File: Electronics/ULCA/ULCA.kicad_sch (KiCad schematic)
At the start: 0 parts

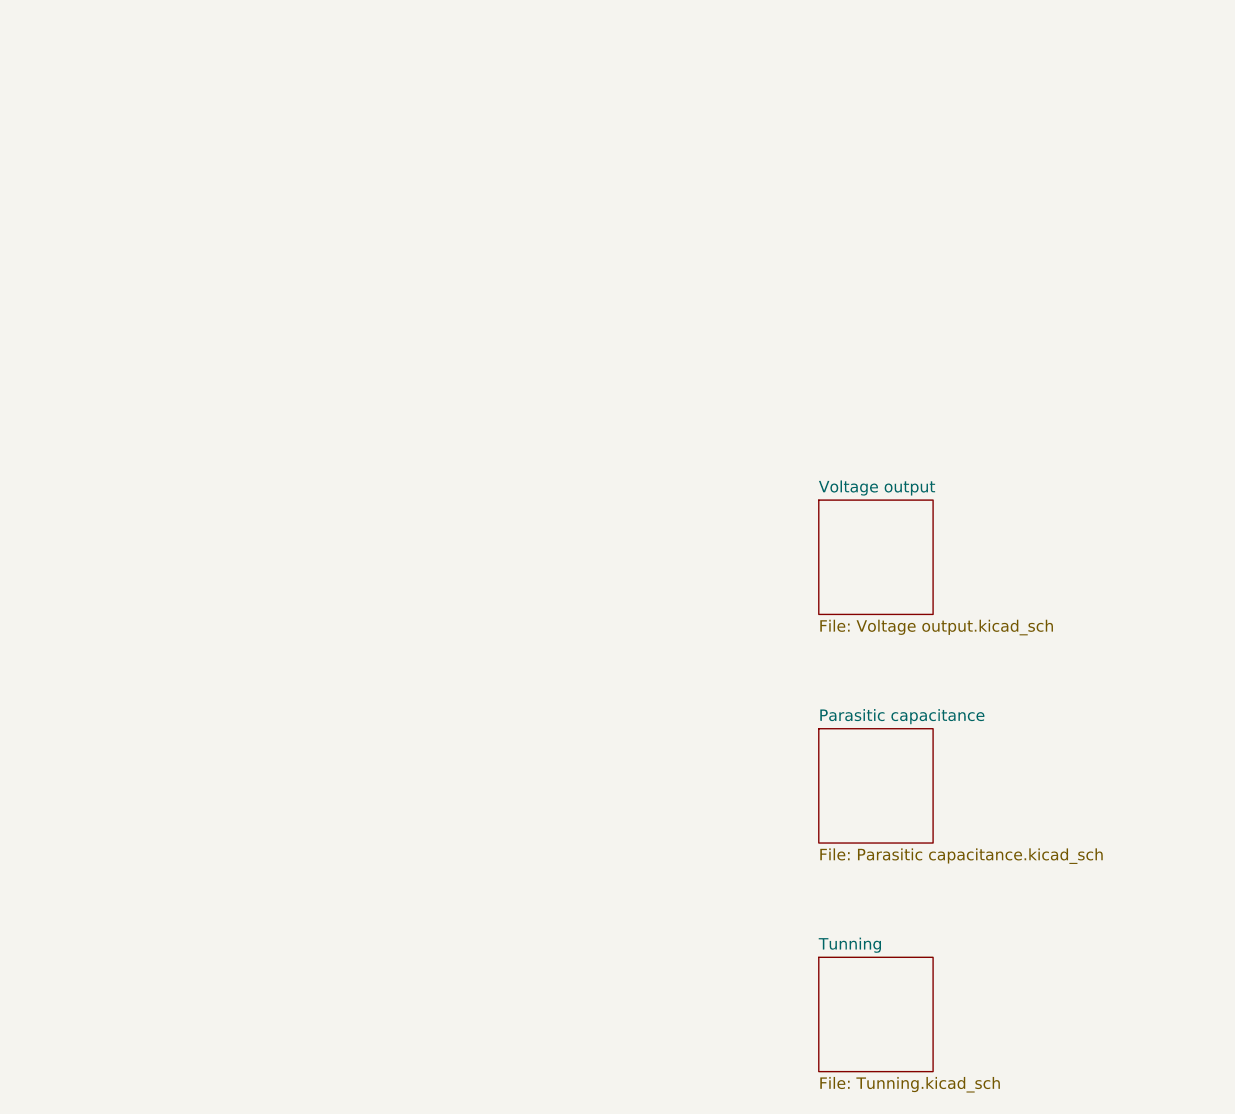
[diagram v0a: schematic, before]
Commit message: Create an okayish tunned ULCA
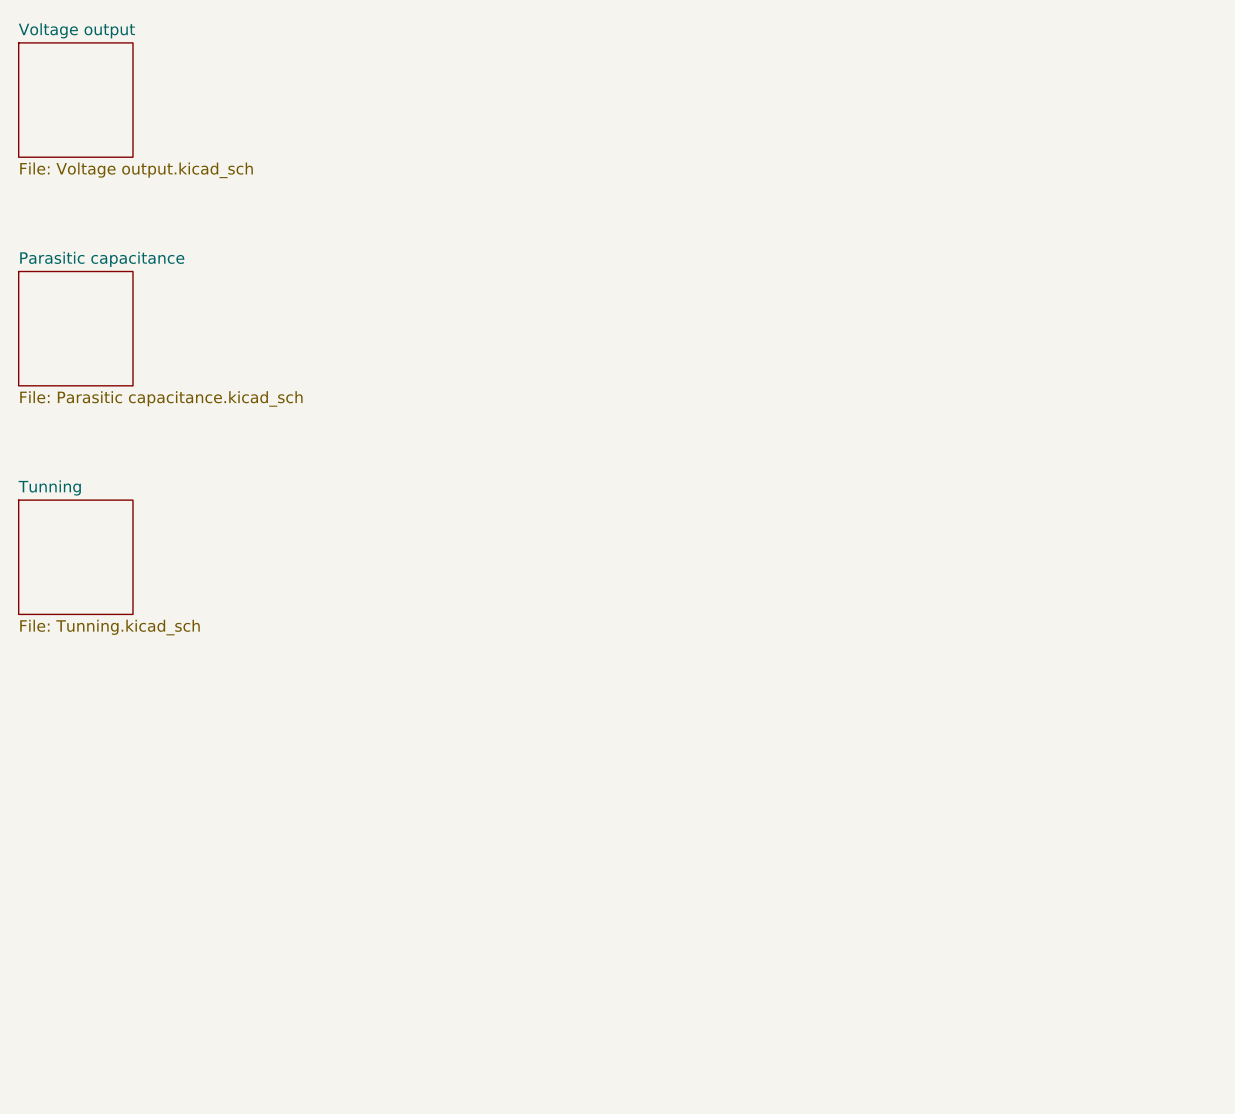
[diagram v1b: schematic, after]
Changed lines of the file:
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@@
 	(paper "A4")
 	(sheet
-		(at 127 139.7)
+		(at 38.1 88.9)
 		(size 12.7 12.7)
 		(exclude_from_sim no)
@@
 		)
 		(property "Sheetname" "Tunning"
-			(at 127 138.9884 0)
+			(at 38.1 88.1884 0)
 			(show_name no)
 			(do_not_autoplace no)
@@
 		)
 		(property "Sheetfile" "Tunning.kicad_sch"
-			(at 127 152.9846 0)
+			(at 38.1 102.1846 0)
 			(show_name no)
 			(do_not_autoplace no)
@@
 	)
 	(sheet
-		(at 127 88.9)
+		(at 38.1 38.1)
 		(size 12.7 12.7)
 		(exclude_from_sim yes)
@@
 		)
 		(property "Sheetname" "Voltage output"
-			(at 127 88.1884 0)
+			(at 38.1 37.3884 0)
 			(show_name no)
 			(do_not_autoplace no)
@@
 		)
 		(property "Sheetfile" "Voltage output.kicad_sch"
-			(at 127 102.1846 0)
+			(at 38.1 51.3846 0)
 			(show_name no)
 			(do_not_autoplace no)
@@
 	)
 	(sheet
-		(at 127 114.3)
+		(at 38.1 63.5)
 		(size 12.7 12.7)
 		(exclude_from_sim yes)
@@
 		)
 		(property "Sheetname" "Parasitic capacitance"
-			(at 127 113.5884 0)
+			(at 38.1 62.7884 0)
 			(show_name no)
 			(do_not_autoplace no)
@@
 		)
 		(property "Sheetfile" "Parasitic capacitance.kicad_sch"
-			(at 127 127.5846 0)
+			(at 38.1 76.7846 0)
 			(show_name no)
 			(do_not_autoplace no)
